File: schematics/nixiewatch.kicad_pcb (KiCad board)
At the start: 2 copper layers, 43 parts, among them Q1 BC546, Q2 IPU80R1K0CE, Q3 BC546, SW1 SW_Push, U1 NE555P, U2 TPIC6B595, U3 MCP1702-5002E/TO, U4 TPIC6B595, U5 TPIC6B595, U6 ATtiny45V-10P, U7 DS1307+, Y1 32.768kHz 12.5pF

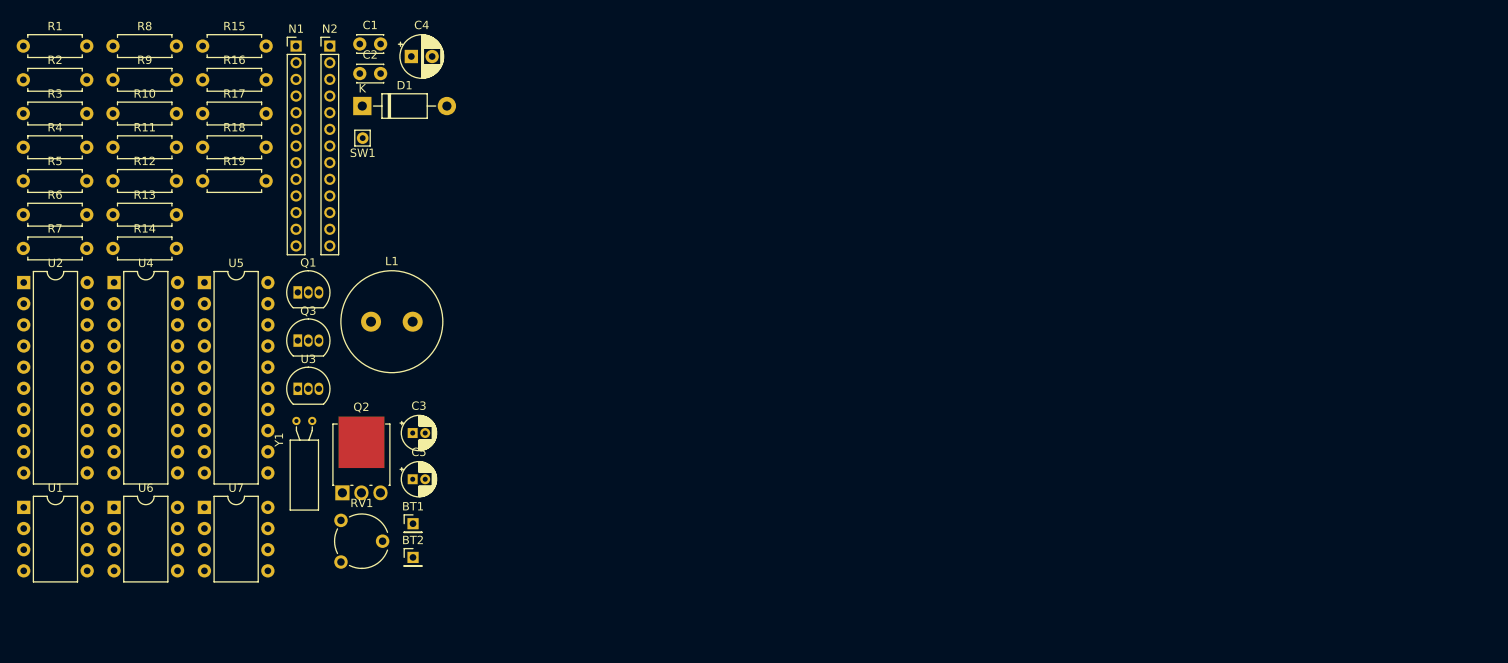
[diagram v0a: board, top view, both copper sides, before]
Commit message: pcb
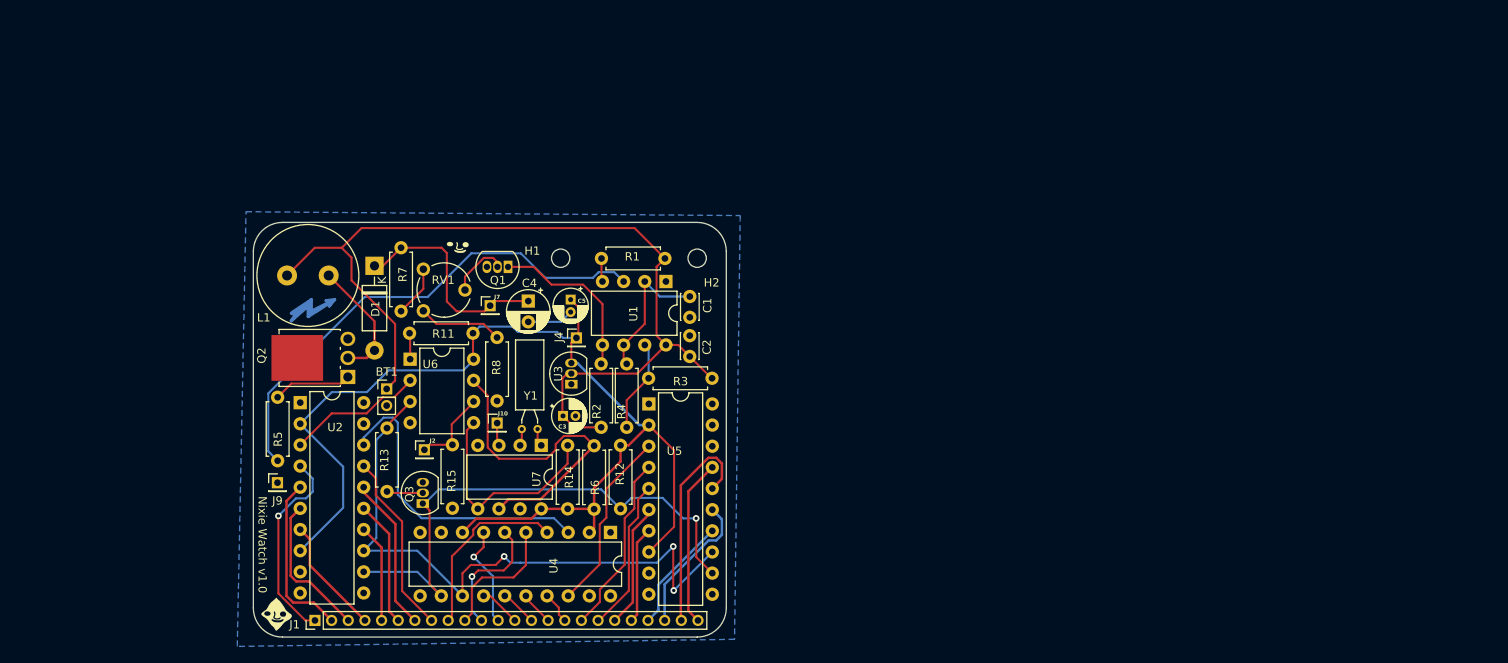
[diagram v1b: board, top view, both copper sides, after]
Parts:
- removed BT2: 3V, Connector_PinHeader_2.00mm:PinHeader_1x01_P2.00mm_Vertical
- removed N1, N2: IN-16, Connector_PinHeader_2.00mm:PinHeader_1x13_P2.00mm_Vertical
- removed R10, R9: 20k, Resistor_THT:R_Axial_DIN0207_L6.3mm_D2.5mm_P7.62mm_Horizontal
- removed R16, R17, R18, R19: 100k, Resistor_THT:R_Axial_DIN0207_L6.3mm_D2.5mm_P7.62mm_Horizontal
- removed SW1: SW_Push, Connector_Pin:Pin_D0.7mm_L6.5mm_W1.8mm_FlatFork
- added G***: LOGO, LOGO, F.Cu at (53.4, 25.4)
- added G***: LOGO, LOGO, F.Cu at (31.5, 69.8)
- added H1: MountingHole, MountingHole:MountingHole_2.2mm_M2, F.Cu at (65.6, 27.0)
- added H2: MountingHole, MountingHole:MountingHole_2.2mm_M2, F.Cu at (82.0, 27.0)
- added J1: Conn_01x25, Connector_PinHeader_2.00mm:PinHeader_1x24_P2.00mm_Vertical, F.Cu at (36.1, 70.5)
- added J10: BT2_3V, Connector_PinHeader_2.00mm:PinHeader_1x01_P2.00mm_Vertical, F.Cu at (58.0, 46.8)
- added J2: ButtonL, Connector_PinHeader_2.00mm:PinHeader_1x01_P2.00mm_Vertical, F.Cu at (49.2, 50.0)
- added J4: ButtonH, Connector_PinHeader_2.00mm:PinHeader_1x01_P2.00mm_Vertical, F.Cu at (67.5, 36.6)
- added J7: ButtonH, Connector_PinHeader_2.00mm:PinHeader_1x01_P2.00mm_Vertical, F.Cu at (57.1, 32.7)
- added J9: BT2GND, Connector_PinHeader_2.00mm:PinHeader_1x01_P2.00mm_Vertical, F.Cu at (31.6, 54.0)
- added REF**: Symbol_Highvoltage_Type1_CopperTop_Small, Symbol:Symbol_Highvoltage_Type1_CopperTop_Small, B.Cu at (36.4, 32.4)
- BT1: footprint Connector_PinHeader_2.00mm:PinHeader_1x01_P2.00mm_Vertical -> Connector_PinHeader_2.00mm:PinHeader_1x02_P2.00mm_Vertical
- moved R3 88.6 mm to (83.8, 41.4), turned to 180 degrees
- moved U1 81.8 mm to (78.2, 29.8), turned to -90 degrees
- moved R1 81.2 mm to (78.1, 27.0), turned to 180 degrees
- moved R2 81.0 mm to (70.5, 47.3), turned to 90 degrees
- moved R4 79.9 mm to (73.5, 47.3), turned to 90 degrees
- moved R6 77.1 mm to (69.6, 57.1), turned to 90 degrees
- moved R12 72.6 mm to (72.8, 57.1), turned to 90 degrees
- moved U4 66.7 mm to (71.6, 59.9), turned to -90 degrees
- moved R15 63.1 mm to (52.6, 57.0), turned to 90 degrees
- moved R14 62.9 mm to (66.5, 57.1), turned to 90 degrees
- moved R8 57.9 mm to (58.0, 36.5), turned to -90 degrees
- moved U5 55.3 mm to (76.2, 44.5)
- moved C2 52.2 mm to (81.1, 38.8), turned to 90 degrees
- moved C1 49.9 mm to (81.1, 31.6), turned to -90 degrees
- moved R13 46.8 mm to (44.8, 55.0), turned to 90 degrees
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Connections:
- net Net-(D1-A) renamed /170V_int
- net Net-(Q3-C) renamed /RCK
- net Net-(U2-SER_IN) renamed /SERIAL_DATA
- net Net-(U2-SRCK) renamed /SRCK
- net Net-(U2-VCC) renamed +5V
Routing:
- net +5V: track 0.00 -> 131.9 mm
- net +BATT: track 0.00 -> 111.5 mm
- net /SRCK: track 0.00 -> 76.1 mm, vias 0 -> 3
- net /RCK: track 0.00 -> 66.0 mm, vias 0 -> 1
- net Net-(U1-Q): track 0.00 -> 60.2 mm
- net Net-(U6-PB2): track 0.00 -> 38.6 mm
- net Net-(U2-SER_OUT): track 0.00 -> 37.2 mm
- net +170V: track 0.00 -> 26.5 mm
- net Net-(U6-AREF/PB0): track 0.00 -> 26.3 mm
- net Net-(J1-Pin_23): track 0.00 -> 26.3 mm
- net Net-(J1-Pin_1): track 0.00 -> 24.1 mm, vias 0 -> 1
- net Net-(U4-SER_OUT): track 0.00 -> 22.0 mm
- net Net-(J1-Pin_8): track 0.00 -> 21.9 mm
- net Net-(J1-Pin_9): track 0.00 -> 21.8 mm
- net Net-(J1-Pin_17): track 0.00 -> 21.7 mm
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- added copper zone on B.Cu, net GND
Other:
- board outline added: 56.8 x 49.8 mm
- board text added: "Nixie Watch v1.0"

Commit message: smd version
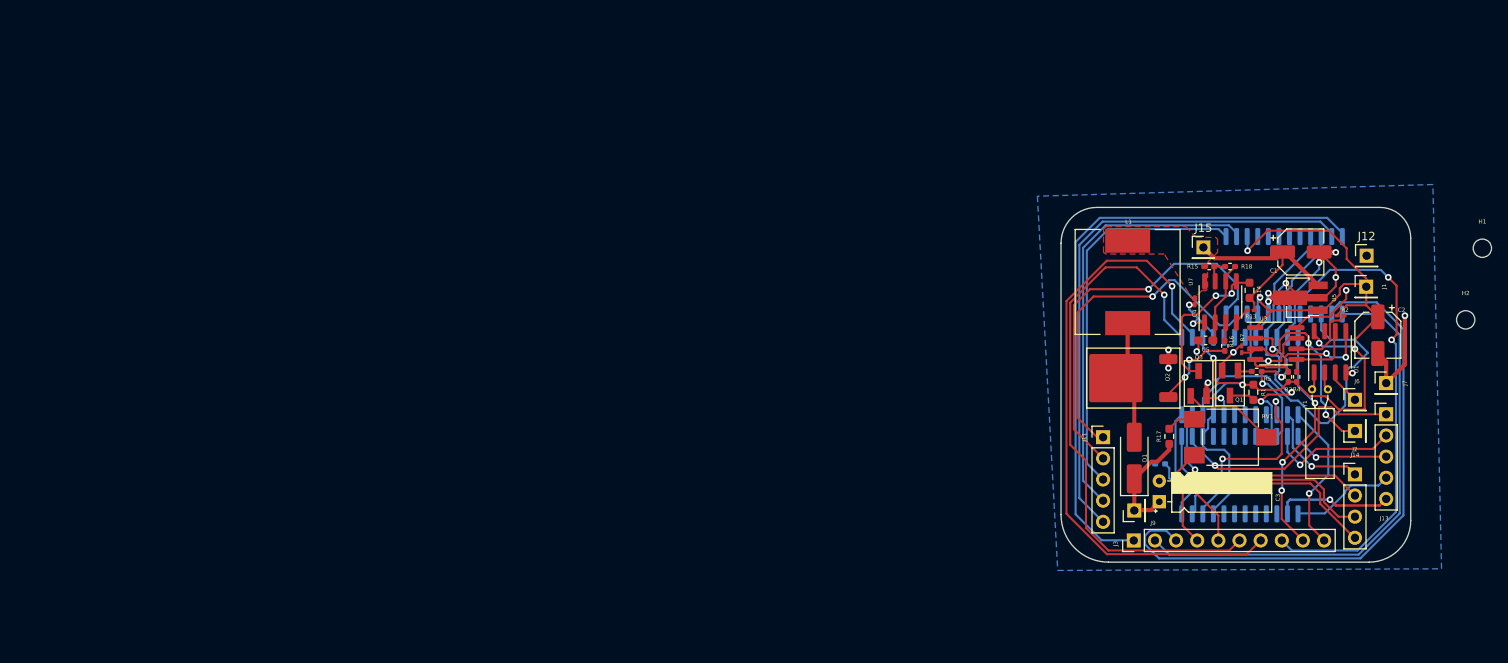
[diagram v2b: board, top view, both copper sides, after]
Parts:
- removed BT1: 8.4V, Connector_PinHeader_2.00mm:PinHeader_1x02_P2.00mm_Vertical
- removed G*** (x2): LOGO, LOGO
- removed J10: BT2_3V, Connector_PinHeader_2.00mm:PinHeader_1x01_P2.00mm_Vertical
- removed J4: ButtonH, Connector_PinHeader_2.00mm:PinHeader_1x01_P2.00mm_Vertical
- removed R11: 10k, Resistor_THT:R_Axial_DIN0207_L6.3mm_D2.5mm_P7.62mm_Horizontal
- removed R12: 47k, Resistor_THT:R_Axial_DIN0207_L6.3mm_D2.5mm_P7.62mm_Horizontal
- removed R6: 2k2, Resistor_THT:R_Axial_DIN0207_L6.3mm_D2.5mm_P7.62mm_Horizontal
- removed R8: 470, Resistor_THT:R_Axial_DIN0207_L6.3mm_D2.5mm_P7.62mm_Horizontal
- removed REF**: Symbol_Highvoltage_Type1_CopperTop_Small, Symbol:Symbol_Highvoltage_Type1_CopperTop_Small
- added J11: Conn_01x05, Connector_PinHeader_2.54mm:PinHeader_1x05_P2.54mm_Vertical, F.Cu at (130.8, 48.5)
- added J12: BTGND, Connector_PinHeader_2.54mm:PinHeader_1x01_P2.54mm_Vertical, F.Cu at (162.4, 26.7)
- added J13: Conn_01x05, Connector_PinHeader_2.54mm:PinHeader_1x05_P2.54mm_Vertical, F.Cu at (164.8, 45.8)
- added J14: Conn_01x04, Connector_PinHeader_2.54mm:PinHeader_1x04_P2.54mm_Vertical, F.Cu at (161.0, 53.0)
- added J15: BT1_8V, Connector_PinHeader_2.54mm:PinHeader_1x01_P2.54mm_Vertical, F.Cu at (142.8, 25.7)
- added J3: Conn_01x10, Connector_PinHeader_2.54mm:PinHeader_1x10_P2.54mm_Vertical, F.Cu at (134.4, 60.9)
- added J6: BT2_3V, Connector_PinHeader_2.54mm:PinHeader_1x01_P2.54mm_Vertical, F.Cu at (161.0, 44.0)
- added R16: 100, Resistor_SMD:R_0402_1005Metric_Pad0.72x0.64mm_HandSolder, F.Cu at (145.4, 37.5)
- added R17: 680k, Resistor_SMD:R_0603_1608Metric_Pad0.98x0.95mm_HandSolder, F.Cu at (138.7, 48.4)
- added R18: 10k, Resistor_SMD:R_0402_1005Metric_Pad0.72x0.64mm_HandSolder, F.Cu at (146.0, 28.0)
- added R19: 470, Resistor_SMD:R_0402_1005Metric_Pad0.72x0.64mm_HandSolder, B.Cu at (137.6, 51.7)
- C1: value 2n2 -> 33u; footprint Capacitor_THT:C_Disc_D3.0mm_W2.0mm_P2.50mm -> Capacitor_SMD:CP_Elec_5x5.3
- C2: value 100n -> 33u; footprint Capacitor_THT:C_Disc_D3.0mm_W2.0mm_P2.50mm -> Capacitor_SMD:CP_Elec_5x5.3
- C3: value 33u -> 1u 200V; footprint Capacitor_THT:CP_Radial_D4.0mm_P1.50mm -> Library:CP_RADIAL_D5.00mm_P2.50mm_H12.0mm_Horizontal
- C4: value 1u 200V -> 100n; footprint Capacitor_THT:CP_Radial_D5.0mm_P2.50mm -> Capacitor_SMD:C_0201_0603Metric_Pad0.64x0.40mm_HandSolder
- C5: value 33u -> 2n4; footprint Capacitor_THT:CP_Radial_D4.0mm_P1.50mm -> Capacitor_SMD:C_0603_1608Metric_Pad1.08x0.95mm_HandSolder
- D1: value 1N4007 -> S1K; footprint Diode_THT:D_DO-41_SOD81_P10.16mm_Horizontal -> Diode_SMD:D_SMA_Handsoldering
- J1: value Conn_01x25 -> ButtonH; footprint Connector_PinHeader_2.00mm:PinHeader_1x24_P2.00mm_Vertical -> Connector_PinHeader_2.54mm:PinHeader_1x01_P2.54mm_Vertical
- J2: footprint Connector_PinHeader_2.00mm:PinHeader_1x01_P2.00mm_Vertical -> Connector_PinHeader_2.54mm:PinHeader_1x01_P2.54mm_Vertical
- J7: value ButtonH -> BT2GND; footprint Connector_PinHeader_2.00mm:PinHeader_1x01_P2.00mm_Vertical -> Connector_PinHeader_2.54mm:PinHeader_1x01_P2.54mm_Vertical
- J9: value BT2GND -> ButtonH; footprint Connector_PinHeader_2.00mm:PinHeader_1x01_P2.00mm_Vertical -> Connector_PinHeader_2.54mm:PinHeader_1x01_P2.54mm_Vertical
- L1: footprint Inductor_THT:L_Radial_D12.0mm_P5.00mm_Neosid_SD12k_style2 -> Inductor_SMD:L_12x12mm_H8mm
- Q1, Q3: value BC546 -> BC846A; footprint Package_TO_SOT_THT:TO-92_Inline -> PCM_Package_TO_SOT_SMD_AKL:SOT-23_Handsoldering
- Q2: value IPU80R1K0CE -> WMO10N60C2; footprint Package_TO_SOT_THT:SIPAK-1EP_Horizontal_TabDown -> PCM_Package_TO_SOT_SMD_AKL:TO-252-2
- R1: value 20k -> 51k; footprint Resistor_THT:R_Axial_DIN0207_L6.3mm_D2.5mm_P7.62mm_Horizontal -> Resistor_SMD:R_0603_1608Metric_Pad0.98x0.95mm_HandSolder
- R13: value 6k8 -> 20k; footprint Resistor_THT:R_Axial_DIN0207_L6.3mm_D2.5mm_P7.62mm_Horizontal -> Resistor_SMD:R_0201_0603Metric_Pad0.64x0.40mm_HandSolder
- R14: value 2k2 -> 51k; footprint Resistor_THT:R_Axial_DIN0207_L6.3mm_D2.5mm_P7.62mm_Horizontal -> Resistor_SMD:R_0603_1608Metric_Pad0.98x0.95mm_HandSolder
- R15: value 20k -> 1k; footprint Resistor_THT:R_Axial_DIN0207_L6.3mm_D2.5mm_P7.62mm_Horizontal -> Resistor_SMD:R_0402_1005Metric_Pad0.72x0.64mm_HandSolder
- R2: value 51k -> 20k; footprint Resistor_THT:R_Axial_DIN0207_L6.3mm_D2.5mm_P7.62mm_Horizontal -> Resistor_SMD:R_0201_0603Metric_Pad0.64x0.40mm_HandSolder
- R3: value 1k -> 2k2; footprint Resistor_THT:R_Axial_DIN0207_L6.3mm_D2.5mm_P7.62mm_Horizontal -> Resistor_SMD:R_0402_1005Metric_Pad0.72x0.64mm_HandSolder
- R4: value 10k -> 2k2; footprint Resistor_THT:R_Axial_DIN0207_L6.3mm_D2.5mm_P7.62mm_Horizontal -> Resistor_SMD:R_0402_1005Metric_Pad0.72x0.64mm_HandSolder
- R5: value 100 -> 6k8; footprint Resistor_THT:R_Axial_DIN0207_L6.3mm_D2.5mm_P7.62mm_Horizontal -> Resistor_SMD:R_0402_1005Metric_Pad0.72x0.64mm_HandSolder
- R7: value 680k -> 20k; footprint Resistor_THT:R_Axial_DIN0207_L6.3mm_D2.5mm_P7.62mm_Horizontal -> Resistor_SMD:R_0201_0603Metric_Pad0.64x0.40mm_HandSolder
- RV1: footprint Potentiometer_THT:Potentiometer_Piher_PT-6-V_Vertical -> Potentiometer_SMD:Potentiometer_ACP_CA6-VSMD_Vertical
- U1: value NE555P -> DS1307Z+; footprint Package_DIP:DIP-8_W7.62mm -> Package_SO:SOIC-8_3.9x4.9mm_P1.27mm
- U2, U4: value TPIC6B595 -> TPIC6A595DWR; footprint Package_DIP:DIP-20_W7.62mm -> Package_SO:SOIC-24W_7.5x15.4mm_P1.27mm; moved to B.Cu
- U3: value MCP1702-5002E/TO -> ATtiny412-SS; footprint Package_TO_SOT_THT:TO-92_Inline -> Package_SO:SOIC-8_3.9x4.9mm_P1.27mm
- U5: value TPIC6B595 -> DI78M05UAB; footprint Package_DIP:DIP-20_W7.62mm -> Package_TO_SOT_SMD:SOT-89-3_Handsoldering
- U6: value ATtiny45V-10P -> TPIC6A595DWR; footprint Package_DIP:DIP-8_W7.62mm -> Package_SO:SOIC-24W_7.5x15.4mm_P1.27mm; moved to B.Cu
- U7: value DS1307+ -> NE555D; footprint Package_DIP:DIP-8_W7.62mm -> Package_SO:SOIC-8_3.9x4.9mm_P1.27mm
- moved J1 132.5 mm to (162.4, 30.4), turned to 0 degrees
- moved U2 119.2 mm to (152.5, 29.1), turned to -90 degrees
- moved R5 117.6 mm to (149.2, 40.6), turned to 0 degrees
- moved J2 111.8 mm to (161.0, 47.8), turned to 90 degrees
- moved H1 110.7 mm to (176.3, 25.8)
- moved J7 108.0 mm to (164.8, 42.0)
- moved R13 106.0 mm to (148.5, 33.2), turned to 180 degrees
- moved J9 103.0 mm to (134.5, 57.3), turned to 90 degrees
- moved R7 101.7 mm to (147.4, 37.9)
- moved L1 101.0 mm to (133.7, 29.9), turned to -90 degrees
- moved U6 100.6 mm to (147.2, 53.0), turned to -90 degrees
- moved RV1 98.1 mm to (146.0, 48.5)
- moved R15 95.4 mm to (143.5, 28.0), turned to 0 degrees
- moved Q2 94.3 mm to (134.4, 41.4), turned to 180 degrees
- moved Q3 94.3 mm to (142.2, 42.0)
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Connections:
- C1 pad 1: Net-(U1-THR) -> +BATT
- C2 pad 1: +BATT -> +5V
- C3 pad 1: +BATT -> +170V
- C4 pad 1: +170V -> +BATT
- C5 pad 1: +5V -> Net-(U7-THR)
- J1 pad 1: Net-(J1-Pin_1) -> +5V
- J7 pad 1: +170V -> GND
- J9 pad 1: GND -> +170V
- Q1 pad 1: Net-(Q1-C) -> Net-(Q1-B)
- Q1 pad 2: Net-(Q1-B) -> GND
- Q1 pad 3: GND -> /RCK
- Q3 pad 1: /RCK -> Net-(Q3-B)
- Q3 pad 2: Net-(Q3-B) -> GND
- Q3 pad 3: GND -> Net-(Q3-C)
- R1 pad 1: +BATT -> /RCK
- R1 pad 2: Net-(U1-R) -> +5V
- R13 pad 1: Net-(Q3-B) -> +BATT
- R13 pad 2: /SRCK -> Net-(U7-R)
- R14 pad 1: +5V -> +BATT
- R14 pad 2: Net-(U6-AREF/PB0) -> Net-(Q3-C)
- R15 pad 1: GND -> +BATT
- R15 pad 2: Net-(J2-Pin_1) -> Net-(U7-DIS)
- R2 pad 1: +BATT -> Net-(U3-~{RESET}/PA0)
- R2 pad 2: Net-(Q1-C) -> +5V
- R3 pad 1: +BATT -> +5V
- R3 pad 2: Net-(U1-DIS) -> Net-(U1-SDA)
- R4 pad 1: Net-(U1-DIS) -> +5V
- R4 pad 2: Net-(U1-THR) -> Net-(U1-SCL)
- R5 pad 1: Net-(Q2-G) -> Net-(Q1-B)
- R5 pad 2: Net-(U1-Q) -> /SRCK
- R7 pad 1: +170V -> GND
- R7 pad 2: Net-(R7-Pad2) -> Net-(J2-Pin_1)
- RV1 pad 2: Net-(Q1-B) -> Net-(Q3-B)
- RV1 pad 3: Net-(R7-Pad2) -> Net-(R17-Pad2)
- U1 pad 1: GND -> Net-(U1-X1)
- U1 pad 2: Net-(U1-THR) -> Net-(U1-X2)
- U1 pad 3: Net-(U1-Q) -> +3V0
- U1 pad 4: Net-(U1-R) -> GND
- U1 pad 5: Net-(Q1-C) -> Net-(U1-SDA)
- U1 pad 6: Net-(U1-THR) -> Net-(U1-SCL)
- U1 pad 7: Net-(U1-DIS) -> unconnected-(U1-SQW/OUT-Pad7)
- U1 pad 8: +BATT -> +5V
- U2 pad 1: unconnected-(U2-NC-Pad1) -> Net-(J11-Pin_3)
- U2 pad 10: GND -> /SRCK
- U2 pad 11: GND -> Net-(J11-Pin_5)
- U2 pad 12: /RCK -> Net-(J3-Pin_1)
- U2 pad 13: /SRCK -> Net-(J3-Pin_2)
- U2 pad 14: Net-(J1-Pin_5) -> Net-(J3-Pin_3)
- U2 pad 15: Net-(J1-Pin_6) -> Net-(U2-SER_OUT)
- U2 pad 16: Net-(J1-Pin_7) -> GND
- U2 pad 17: Net-(J1-Pin_8) -> GND
- U2 pad 18: Net-(U2-SER_OUT) -> GND
- U2 pad 2: +5V -> Net-(J11-Pin_4)
- U2 pad 20: unconnected-(U2-NC-Pad20) -> GND
- U2 pad 3: /SERIAL_DATA -> +5V
- U2 pad 4: Net-(J1-Pin_1) -> GND
- U2 pad 5: Net-(J1-Pin_2) -> GND
- U2 pad 6: Net-(J1-Pin_3) -> GND
- U2 pad 7: Net-(J1-Pin_4) -> GND
- U2 pad 8: +5V -> GND
- U2 pad 9: GND -> /RCK
- U3 pad 1: GND -> +5V
- U3 pad 2: +BATT -> /SRCK
- U3 pad 3: +5V -> Net-(J2-Pin_1)
- U4 pad 1: unconnected-(U4-NC-Pad1) -> Net-(J3-Pin_6)
- U4 pad 10: GND -> /SRCK
- U4 pad 11: GND -> Net-(J3-Pin_8)
- U4 pad 12: /RCK -> Net-(J3-Pin_9)
- U4 pad 13: /SRCK -> Net-(J3-Pin_10)
- U4 pad 14: Net-(J1-Pin_13) -> Net-(J14-Pin_1)
- U4 pad 15: Net-(J1-Pin_14) -> Net-(U4-SER_OUT)
- U4 pad 16: Net-(J1-Pin_15) -> GND
- U4 pad 17: Net-(J1-Pin_16) -> GND
- U4 pad 18: Net-(U4-SER_OUT) -> GND
- U4 pad 2: +5V -> Net-(J3-Pin_7)
- U4 pad 20: unconnected-(U4-NC-Pad20) -> GND
- U4 pad 3: Net-(U2-SER_OUT) -> +5V
- U4 pad 4: Net-(J1-Pin_9) -> GND
- U4 pad 5: Net-(J1-Pin_10) -> GND
- U4 pad 6: Net-(J1-Pin_11) -> GND
- U4 pad 7: Net-(J1-Pin_12) -> GND
- U4 pad 8: +5V -> GND
- U4 pad 9: GND -> /RCK
- U5 pad 1: unconnected-(U5-NC-Pad1) -> +5V
- U5 pad 2: +5V -> GND
- U5 pad 3: Net-(U4-SER_OUT) -> +BATT
- U6 pad 2: /SERIAL_DATA -> Net-(J13-Pin_1)
- U6 pad 3: /SRCK -> +5V
- U6 pad 5: Net-(U6-AREF/PB0) -> GND
- U6 pad 6: Net-(J2-Pin_1) -> GND
- U6 pad 7: Net-(U6-PB2) -> GND
- U6 pad 8: +5V -> GND
- U7 pad 1: Net-(U7-X1) -> GND
- U7 pad 2: Net-(U7-X2) -> Net-(U7-THR)
- U7 pad 3: +3V0 -> Net-(U7-Q)
- U7 pad 4: GND -> Net-(U7-R)
- U7 pad 5: Net-(U6-AREF/PB0) -> Net-(Q3-C)
- U7 pad 6: Net-(U6-PB2) -> Net-(U7-THR)
- U7 pad 7: unconnected-(U7-SQW/OUT-Pad7) -> Net-(U7-DIS)
- U7 pad 8: +5V -> +BATT
- Y1 pad 1: Net-(U7-X1) -> Net-(U1-X1)
- Y1 pad 2: Net-(U7-X2) -> Net-(U1-X2)
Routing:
- net +BATT: track 111.5 -> 25.2 mm
- net GND: track 5.58 -> 91.7 mm, vias 0 -> 17
- net Net-(J3-Pin_1): track 0.00 -> 75.4 mm
- net Net-(J3-Pin_7): track 0.00 -> 74.7 mm, vias 0 -> 1
- net Net-(J3-Pin_3): track 0.00 -> 72.5 mm
- net Net-(J3-Pin_6): track 0.00 -> 68.3 mm, vias 0 -> 1
- net Net-(J11-Pin_5): track 0.00 -> 66.9 mm
- net Net-(J3-Pin_8): track 0.00 -> 62.8 mm, vias 0 -> 2
- net Net-(J3-Pin_2): track 0.00 -> 61.6 mm
- net Net-(U1-Q): track 60.2 -> 0.00 mm
- net Net-(J11-Pin_4): track 0.00 -> 51.9 mm
- net Net-(J11-Pin_2): track 0.00 -> 46.7 mm, vias 0 -> 1
- net Net-(J11-Pin_3): track 0.00 -> 46.5 mm
- net Net-(J11-Pin_1): track 0.00 -> 40.4 mm, vias 0 -> 1
- net /SRCK: track 76.1 -> 35.7 mm
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- added copper zone on F.Cu, net +BATT
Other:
- board size 56.8 x 49.8 mm -> 42 x 42.6 mm
- board text removed: "Nixie Watch v1.0"
